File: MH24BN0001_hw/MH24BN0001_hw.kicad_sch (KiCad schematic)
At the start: 1 part, among them J1 ST-Link V2 Header

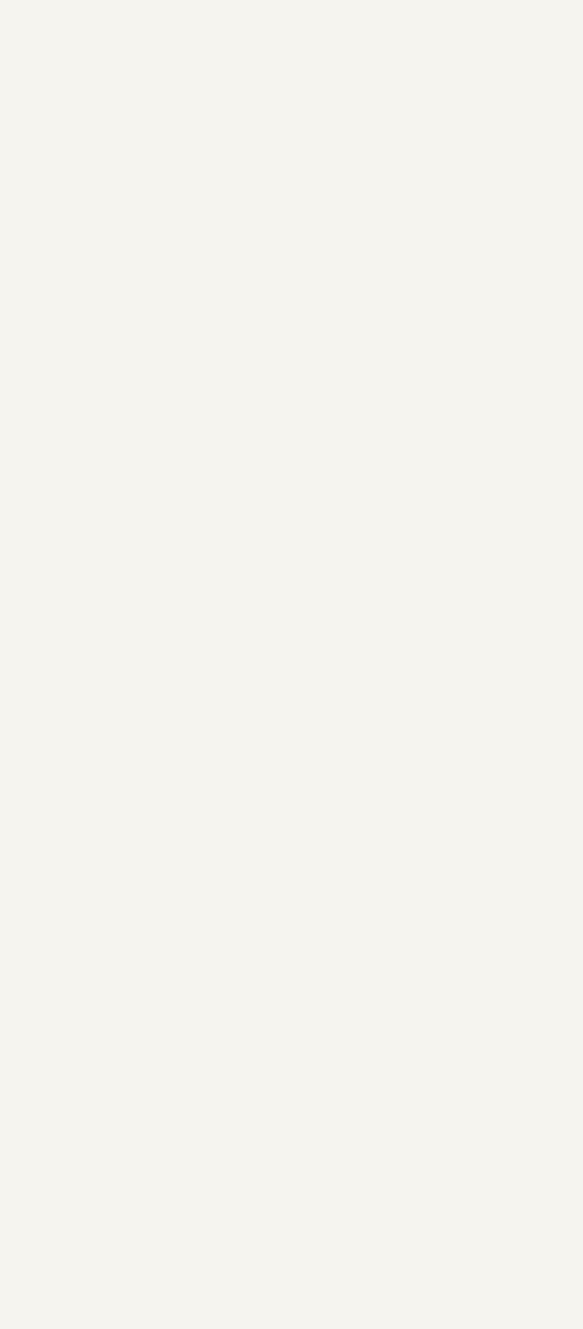
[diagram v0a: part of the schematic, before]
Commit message: previous commit
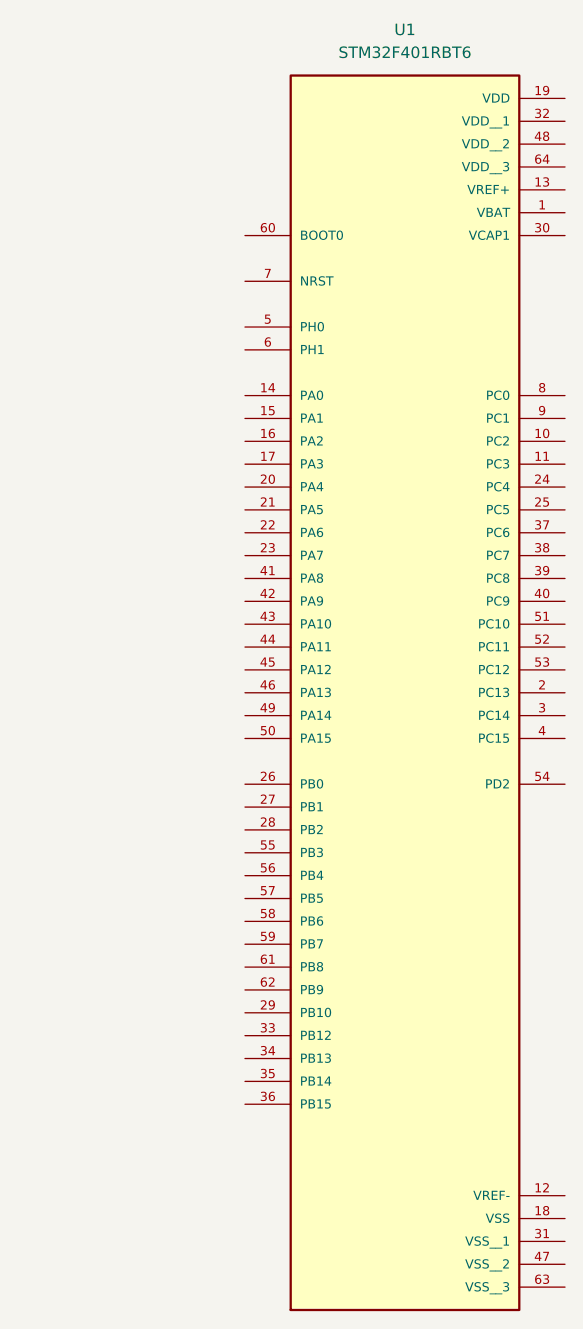
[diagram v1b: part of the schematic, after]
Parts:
- added U1: STM32F401RBT6, Library:QFP50P1200X1200X160-64N, symbol Sym_lib:STM32F401RBT6
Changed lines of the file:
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@@
+	)
+	(symbol
+		(lib_id "Sym_lib:STM32F401RBT6")
+		(at 218.44 92.71 0)
+		(unit 1)
+		(exclude_from_sim no)
+		(in_bom yes)
+		(on_board yes)
+		(dnp no)
+		(fields_autoplaced yes)
+		(property "Reference" "U1"
+			(at 218.44 16.51 0)
+			(effects
+				(font
+					(size 1.27 1.27)
+				)
+			)
+		)
+		(property "Value" "STM32F401RBT6"
+			(at 218.44 19.05 0)
+			(effects
+				(font
+					(size 1.27 1.27)
+				)
+			)
+		)
+		(property "Footprint" "Library:QFP50P1200X1200X160-64N"
+			(at 218.44 92.71 0)
+			(effects
+				(font
+					(size 1.27 1.27)
+				)
+				(justify bottom)
+				(hide yes)
+			)
+		)
+		(property "Datasheet" "https://www.st.com/content/ccc/resource/technical/document/datasheet/9e/50/b1/5a/5f/ae/4d/c1/DM00086815.pdf/files/DM00086815.pdf/jcr:content/translations/en.DM00086815.pdf"
+			(at 218.44 92.71 0)
+			(effects
+				(font
+					(size 1.27 1.27)
+				)
+				(hide yes)
+			)
+		)
+		(property "Description" ""
+			(at 218.44 92.71 0)
+			(effects
+				(font
+					(size 1.27 1.27)
+				)
+				(hide yes)
+			)
+		)
+		(property "MANUFACTURER" "STMicroelectronics"
+			(at 218.44 92.71 0)
+			(effects
+				(font
+					(size 1.27 1.27)
+				)
+				(justify bottom)
+				(hide yes)
+			)
+		)
+		(pin "43"
+		)
+		(pin "44"
+		)
+		(pin "13"
+		)
+		(pin "1"
+		)
+		(pin "11"
+		)
+		(pin "19"
+		)
+		(pin "30"
+		)
+		(pin "33"
+		)
+		(pin "17"
+		)
+		(pin "34"
+		)
+		(pin "2"
+		)
+		(pin "16"
+		)
+		(pin "21"
+		)
+		(pin "3"
+		)
+		(pin "26"
+		)
+		(pin "22"
+		)
+		(pin "27"
+		)
+		(pin "12"
+		)
+		(pin "35"
+		)
+		(pin "36"
+		)
+		(pin "15"
+		)
+		(pin "40"
+		)
+		(pin "37"
+		)
+		(pin "14"
+		)
+		(pin "10"
+		)
+		(pin "41"
+		)
+		(pin "38"
+		)
+		(pin "29"
+		)
+		(pin "24"
+		)
+		(pin "42"
+		)
+		(pin "18"
+		)
+		(pin "23"
+		)
+		(pin "28"
+		)
+		(pin "31"
+		)
+		(pin "32"
+		)
+		(pin "20"
+		)
+		(pin "25"
+		)
+		(pin "39"
+		)
+		(pin "4"
+		)
+		(pin "49"
+		)
+		(pin "52"
+		)
+		(pin "55"
+		)
+		(pin "64"
+		)
+		(pin "9"
+		)
+		(pin "60"
+		)
+		(pin "7"
+		)
+		(pin "62"
+		)
+		(pin "56"
+		)
+		(pin "47"
+		)
+		(pin "63"
+		)
+		(pin "45"
+		)
+		(pin "5"
+		)
+		(pin "50"
+		)
+		(pin "6"
+		)
+		(pin "48"
+		)
+		(pin "46"
+		)
+		(pin "57"
+		)
+		(pin "53"
+		)
+		(pin "8"
+		)
+		(pin "51"
+		)
+		(pin "61"
+		)
+		(pin "58"
+		)
+		(pin "59"
+		)
+		(pin "54"
+		)
+		(instances
+			(project ""
+				(path "/1e9f19f6-5b3f-4aa5-b603-02119a5ead72"
+					(reference "U1")
+					(unit 1)
+				)
+			)
+		)
 	)
 	(symbol
